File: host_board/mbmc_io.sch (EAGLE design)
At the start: 48 parts, among them J1 1-1586043-4, J2 1586044-4

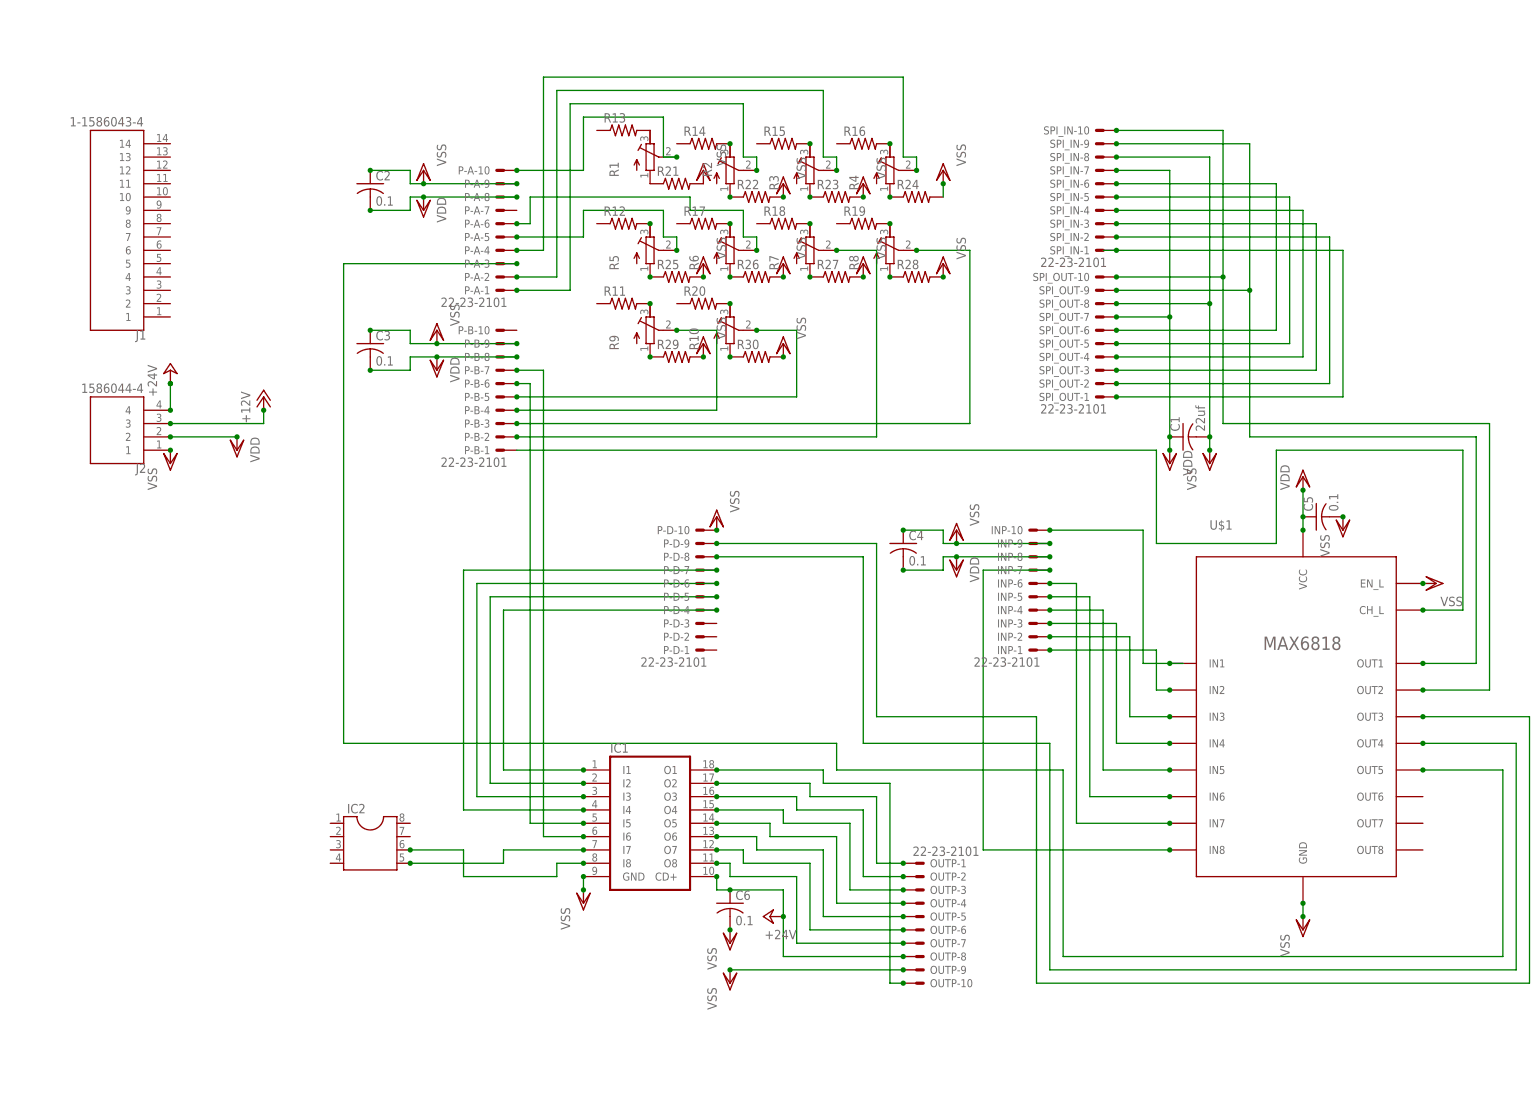
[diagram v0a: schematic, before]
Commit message: up
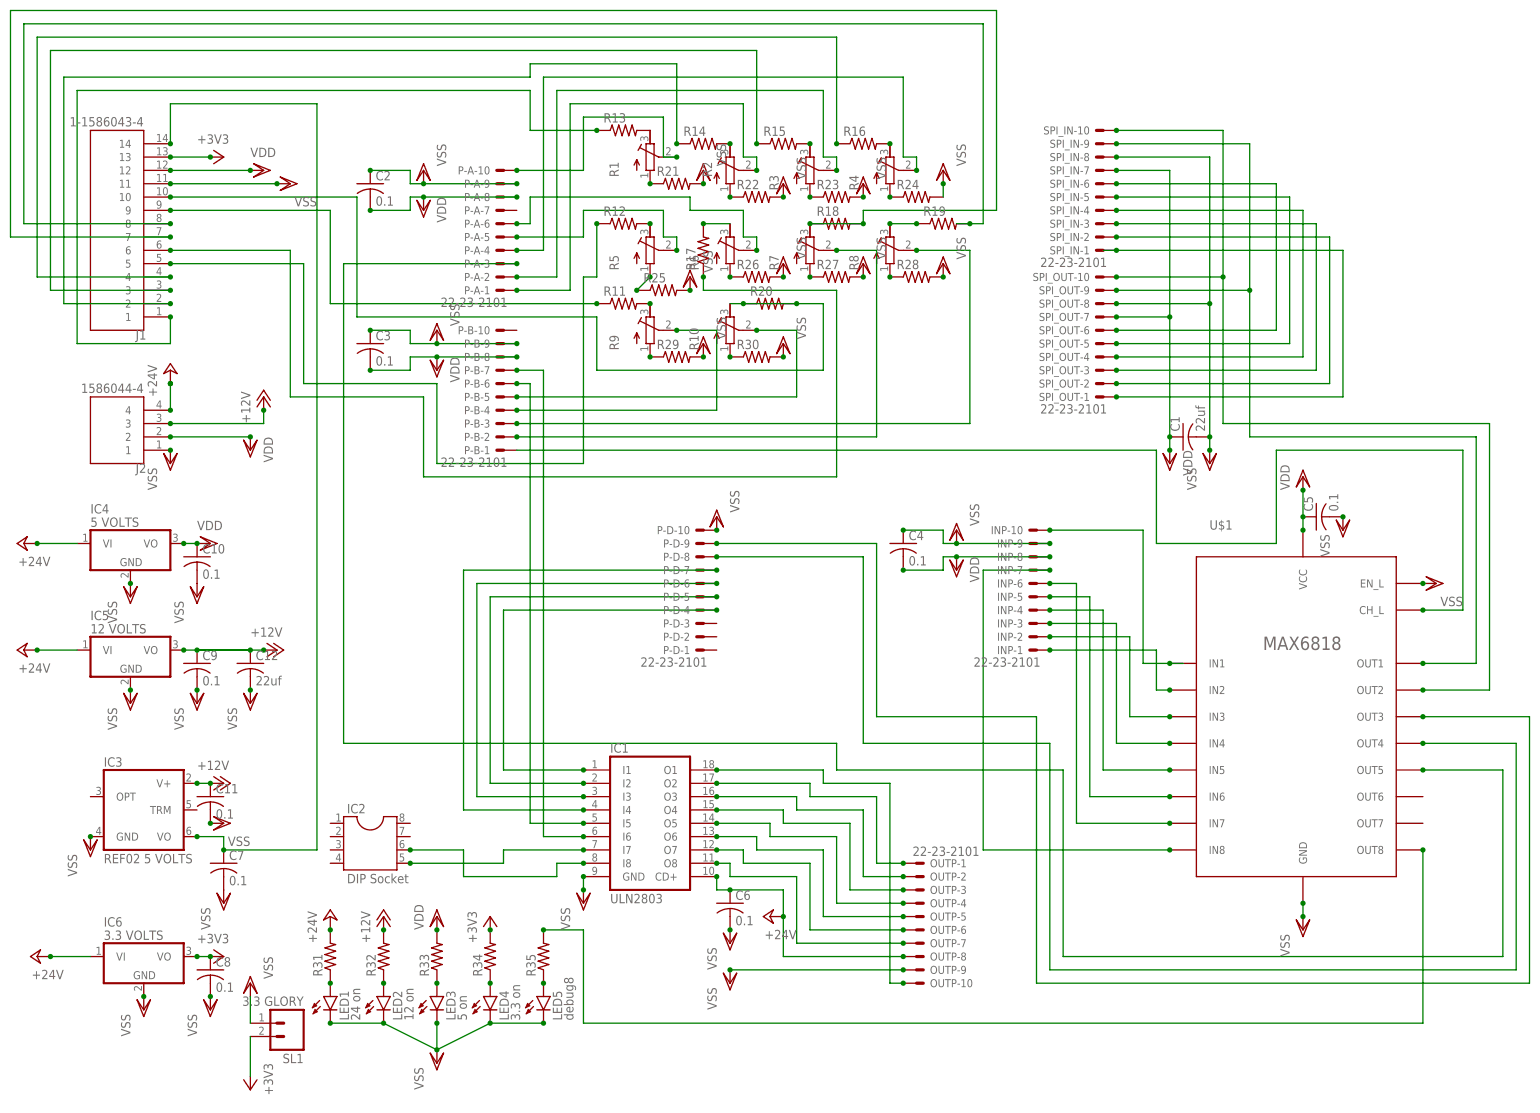
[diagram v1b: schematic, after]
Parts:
- added C10, C11, C7, C8, C9: 0.1, rcl:C-USC0805
- added C12: 22uf, rcl:C-USC0805
- added IC3: REF02 5 VOLTS, linear:REF02Z
- added IC4: 5 VOLTS, linear:7805TV
- added IC5: 12 VOLTS, linear:7805TV
- added IC6: 3.3 VOLTS, linear:7805TV
- added LED1: 24 on, led:LEDCHIPLED_1206
- added LED2: 12 on, led:LEDCHIPLED_1206
- added LED3: 5 on, led:LEDCHIPLED_1206
- added LED4: 3.3 on, led:LEDCHIPLED_1206
- added LED5: debug8, led:LEDCHIPLED_1206
- added R31, R32, R33, R34, R35: (no value), rcl:R-US_R0805
- added SL1: 3.3 GLORY, con-amp-quick:M02
- IC1: value (none) -> ULN2803
- IC2: value (none) -> DIP Socket
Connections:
- new net +3V3: C8.1, IC6.VO, J1.13, R34.2, SL1.2
- new net N$24: J1.2, R14.1
- new net N$61: C7.1, IC3.VO, J1.14
- new net N$68: J1.4, R16.1
- new net N$69: J1.9, R11.1
- new net N$70: J1.3, R15.1
- new net N$71: J1.10, R10.E, R20.1, R20.2
- new net N$72: J1.5, R12.1
- new net N$73: J1.6, R17.1
- new net N$74: J1.1, R13.1
- new net N$76: LED1.A, R31.1
- new net N$77: LED2.A, R32.1
- new net N$78: LED3.A, R33.1
- new net N$79: LED4.A, R34.1
- new net N$80: LED5.A, R35.1
- new net N$81: R35.2, U$1.OUT8
- net +12V: now also C11.1, C12.1, C9.1, IC3.V+, IC5.VO, R32.2
- net +24V: now also IC4.VI, IC5.VI, IC6.VI, R31.2
- net N$10: now also J1.8, R19.2; no longer R10.E, R20.2
- net N$8: now also J1.7, R18.1
- net N$9: now also R19.1; no longer R19.2
- net VDD: now also C10.1, IC4.VO, J1.12, R33.2
- net VSS: now also C10.2, C11.2, C12.2, C7.2, C8.2, C9.2, IC3.GND, IC4.GND, IC5.GND, IC6.GND, J1.11, LED1.C, LED2.C, LED3.C, LED4.C, LED5.C, SL1.1
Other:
- moved on the sheet: R17, R18, R19, R20, R25
